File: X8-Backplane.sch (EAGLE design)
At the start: 15 parts, among them U1 LM2678

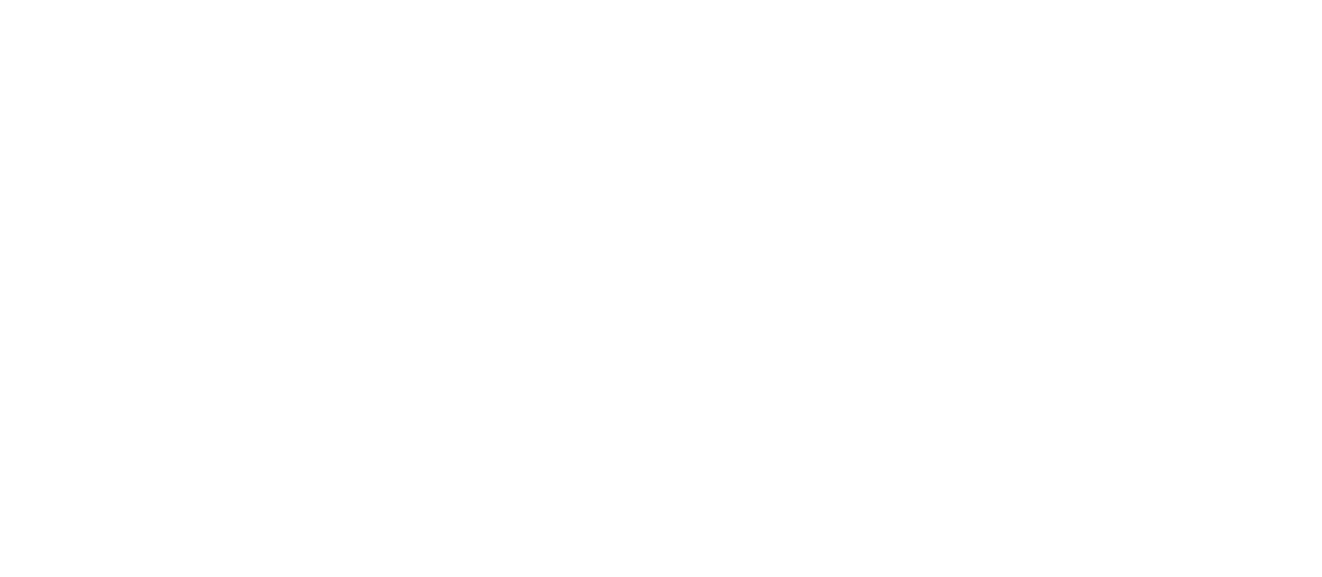
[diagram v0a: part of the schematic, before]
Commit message: because I can
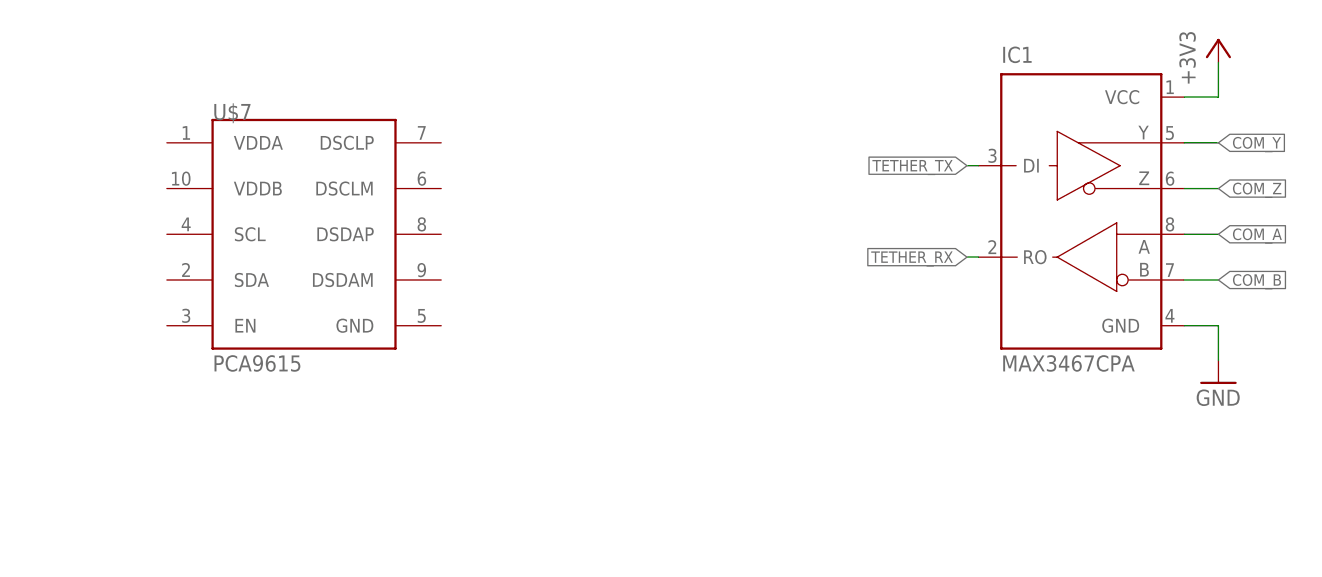
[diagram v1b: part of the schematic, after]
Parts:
- added IC1: MAX3467CPA, maxim:MAX3467CPA
- added U$7: PCA9615, test_lib:PCA9615
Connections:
- new net +3V3: IC1.VCC
- new net COM_A: IC1.A
- new net COM_B: IC1.B
- new net COM_Y: IC1.Y
- new net COM_Z: IC1.Z
- new net TETHER_RX: IC1.RO
- new net TETHER_TX: IC1.DI
- net GND: now also IC1.GND
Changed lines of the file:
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@@
 <part name="U$3" library="Other" deviceset="BNO055_9DOF_BREAKOUT" device=""/>
 <part name="U$4" library="backplane_to_shield_connector" deviceset="SHIELDCONNECTOR" device=""/>
+<part name="IC1" library="maxim" deviceset="MAX3467*" device="PA" technology="C"/>
+<part name="+3V1" library="supply1" deviceset="+3V3" device=""/>
+<part name="GND1" library="supply1" deviceset="GND" device=""/>
+<part name="U$7" library="test_lib" deviceset="PCA9615" device=""/>
 </parts>
 <sheets>
@@
 <instance part="U$4" gate="G$1" x="373.38" y="91.44"/>
 <instance part="U$4" gate="G$2" x="419.1" y="88.9"/>
+<instance part="IC1" gate="G$1" x="496.57" y="172.72"/>
+<instance part="+3V1" gate="G$1" x="513.08" y="191.77"/>
+<instance part="GND1" gate="1" x="513.08" y="153.67"/>
+<instance part="U$7" gate="G$1" x="408.94" y="165.1"/>
 </instances>
 <busses>
@@
 <junction x="68.58" y="-137.16"/>
 </segment>
+<segment>
+<pinref part="IC1" gate="G$1" pin="GND"/>
+<wire x1="509.27" y1="160.02" x2="513.08" y2="160.02" width="0.1524" layer="91"/>
+<wire x1="513.08" y1="160.02" x2="513.08" y2="156.21" width="0.1524" layer="91"/>
+<pinref part="GND1" gate="1" pin="GND"/>
+</segment>
 </net>
 <net name="+12V" class="0">
@@
 </segment>
 </net>
+<net name="+3V3" class="0">
+<segment>
+<pinref part="IC1" gate="G$1" pin="VCC"/>
+<wire x1="509.27" y1="185.42" x2="513.08" y2="185.42" width="0.1524" layer="91"/>
+<wire x1="513.08" y1="185.42" x2="513.08" y2="189.23" width="0.1524" layer="91"/>
+<pinref part="+3V1" gate="G$1" pin="+3V3"/>
+</segment>
+</net>
+<net name="TETHER_RX" class="0">
+<segment>
+<pinref part="IC1" gate="G$1" pin="RO"/>
+<wire x1="486.41" y1="167.64" x2="485.14" y2="167.64" width="0.1524" layer="91"/>
+<label x="485.14" y="167.64" size="1.27" layer="95" rot="R180" xref="yes"/>
+</segment>
+</net>
+<net name="TETHER_TX" class="0">
+<segment>
+<label x="485.14" y="177.8" size="1.27" layer="95" rot="R180" xref="yes"/>
+<pinref part="IC1" gate="G$1" pin="DI"/>
+<wire x1="485.14" y1="177.8" x2="486.41" y2="177.8" width="0.1524" layer="91"/>
+</segment>
+</net>
+<net name="COM_A" class="0">
+<segment>
+<pinref part="IC1" gate="G$1" pin="A"/>
+<wire x1="509.27" y1="170.18" x2="513.08" y2="170.18" width="0.1524" layer="91"/>
+<label x="513.08" y="170.18" size="1.27" layer="95" xref="yes"/>
+</segment>
+</net>
+<net name="COM_B" class="0">
+<segment>
+<pinref part="IC1" gate="G$1" pin="B"/>
+<wire x1="509.27" y1="165.1" x2="513.08" y2="165.1" width="0.1524" layer="91"/>
+<label x="513.08" y="165.1" size="1.27" layer="95" xref="yes"/>
+</segment>
+</net>
+<net name="COM_Y" class="0">
+<segment>
+<pinref part="IC1" gate="G$1" pin="Y"/>
+<wire x1="509.27" y1="180.34" x2="513.08" y2="180.34" width="0.1524" layer="91"/>
+<label x="513.08" y="180.34" size="1.27" layer="95" xref="yes"/>
+</segment>
+</net>
+<net name="COM_Z" class="0">
+<segment>
+<pinref part="IC1" gate="G$1" pin="Z"/>
+<wire x1="509.27" y1="175.26" x2="513.08" y2="175.26" width="0.1524" layer="91"/>
+<label x="513.08" y="175.26" size="1.27" layer="95" xref="yes"/>
+</segment>
+</net>
